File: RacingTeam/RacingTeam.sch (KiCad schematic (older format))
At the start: 68 parts, among them J1 BusIn, J2 PCB OUT, J3 Shutdown Circuit, J5 PreCharge Relay Out, J6 AIR, J7 AIR, J8 Precharge Relay, J9 Discharge Relay, Q1 2N7002, Q2 TP0610T, Q3 2N7002, Q4 TP0610T, Q5 TP0610T, Q6 2N7002, U1 LM311, U11 GLV-, U12 GLV+, U2 4N35, U3 NE555D, U4 GLV+, U5 GLV-, U6 GLV+, U6 LM311, U7 GLV-, U8 GLV-, U9 GLV-

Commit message: Update SPAN02A12.kicad_mod, EC3SAW.STEP, and 8 more files...
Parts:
- removed F1: 1000V 5A, symbol Device:Fuse
- removed J3: Shutdown Circuit, symbol Connector_Generic:Conn_01x02
- removed J8: Precharge Relay, symbol Connector_Generic:Conn_01x02
- removed J9: Discharge Relay, symbol Connector_Generic:Conn_01x02
- removed PS1: SPAN02A-12, Footprints:SPAN02A12, symbol RacingTeamPCB:SPAN02A-12
- removed R24: 2kΩ, Footprints:R_0603_1608Metric, symbol RacingTeamPCB:R
- removed R?: 100Ω, Footprints:R_0603_1608Metric, symbol RacingTeamPCB:R
- added D4, D5, D6: Flyback, symbol Device:D
- added D7: 12V, symbol RacingTeamPCB:D_Zener
- added D7: LED, symbol RacingTeamPCB:LED
- added J3, J4, J8, J9: Conn_01x01, symbol Connector_Generic:Conn_01x01
- added PS1: EC3SAW-24S12P, symbol RacingTeamPCB:EC3SAW-24S12P
- added Q7, Q8: 2N7002, symbol RacingTeamPCB:2N7000
- added R13: 1.2kΩ, symbol RacingTeamPCB:R
- added R18: 22kΩ, symbol RacingTeamPCB:R
- added R28, R29, R30: 0Ω, symbol RacingTeamPCB:R
- added U10: GLV-, symbol RacingTeamPCB:GLV-
- C1, C2, C3, C4, C5, C6, C7, C8: footprint Footprints:C_0603_1608Metric -> (none)
- J6: value AIR -> AIROut
- J7: value AIR -> Discharge Relay Out
- Q1, Q2, Q3, Q4, Q5, Q6: footprint Package_TO_SOT_SMD:SOT-23 -> (none)
- R1, R10, R11, R2, R3, R4, R5, R6, R7, R8, R9: footprint Footprints:R_0603_1608Metric -> (none)
- R12, R25: renamed from R23; footprint Footprints:R_0603_1608Metric -> (none)
- R14: renamed from R12; footprint Footprints:R_0603_1608Metric -> (none)
- R15: renamed from R13; footprint Footprints:R_0603_1608Metric -> (none)
- R16: renamed from R14; footprint Footprints:R_0603_1608Metric -> (none)
- R17: renamed from R15; footprint Footprints:R_0603_1608Metric -> (none)
- R19: renamed from R16; footprint Footprints:R_0603_1608Metric -> (none)
- R20: renamed from R17; footprint Footprints:R_0603_1608Metric -> (none)
- R21: renamed from R20; footprint Footprints:R_0603_1608Metric -> (none)
- R22: renamed from R21; footprint Footprints:R_0603_1608Metric -> (none)
- R23: renamed from R18; footprint Footprints:R_0603_1608Metric -> (none)
- R24: renamed from R19; footprint Footprints:R_0603_1608Metric -> (none)
- R26: renamed from R24; footprint Footprints:R_0603_1608Metric -> (none)
- R27: renamed from R22; footprint Footprints:R_0603_1608Metric -> (none)
- U1: footprint Footprints:TSSOP-8 -> (none)
- U2: footprint Footprints:4N35PDIP-SMD -> (none)
- U3: footprint Footprints:SOIC-8_3.9x4.9mm_P1.27mm -> (none)
- gave numbers to parts that had none: 2
- renumbered U6 to U20
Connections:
- net labels added: AIROR, PreChargeOR
- net labels removed: Discharge+, Discharge-, PrechargeIn
- wire segments 165 -> 173
- no-connect marks 4 -> 3
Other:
- note added: "12V+ - Unconverted 12V from Battery\nVCC - Diode Filtered GLV+\nGLV+ - Grounded Low Voltage +\nGLV- - Grounded Low Voltage -"
- note added: "Discharge Control\n"
- note added: "Drain\nGate\nSource"
- note added: "If=10mA"
- note added: "PreCharge Control\n\n"
- note added: "Source\nGate\nDrain\n"
- note removed: "Discharge"
- note removed: "Logic\n1. Shutdown Circuit Open Car On = Precharge Relay Open\n2. Shutdown Circuit Open Car Off = Precharge Relay Open\n3. Shutdown Circuit Closed Car Off = Precharge Relay Open\n4. Shutdown Circuit Closed Car On = Precharge Relay Closed"
- note removed: "PreCharge and Discharge (Control Side)\n"
- note removed: "Precharge and Discharge Relay (Drive Side)\n"
- note removed: "Shutdown Initiation"
- moved on the sheet: D3, J2, J5, J6, Q5, Q6

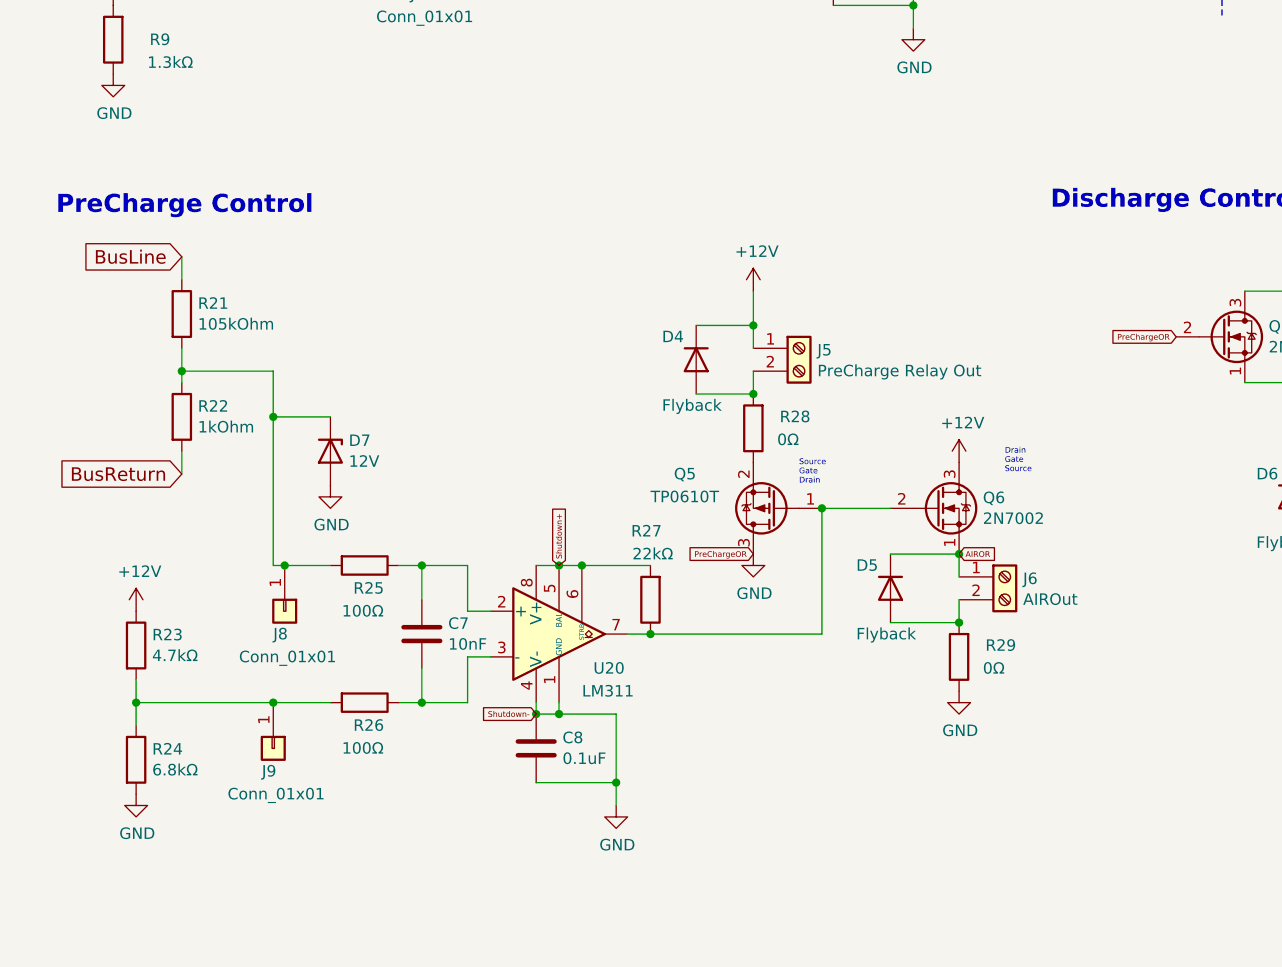
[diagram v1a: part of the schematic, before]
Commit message: Update RacingTeam.zip, PCBBom.xlsx, and 2 more files...
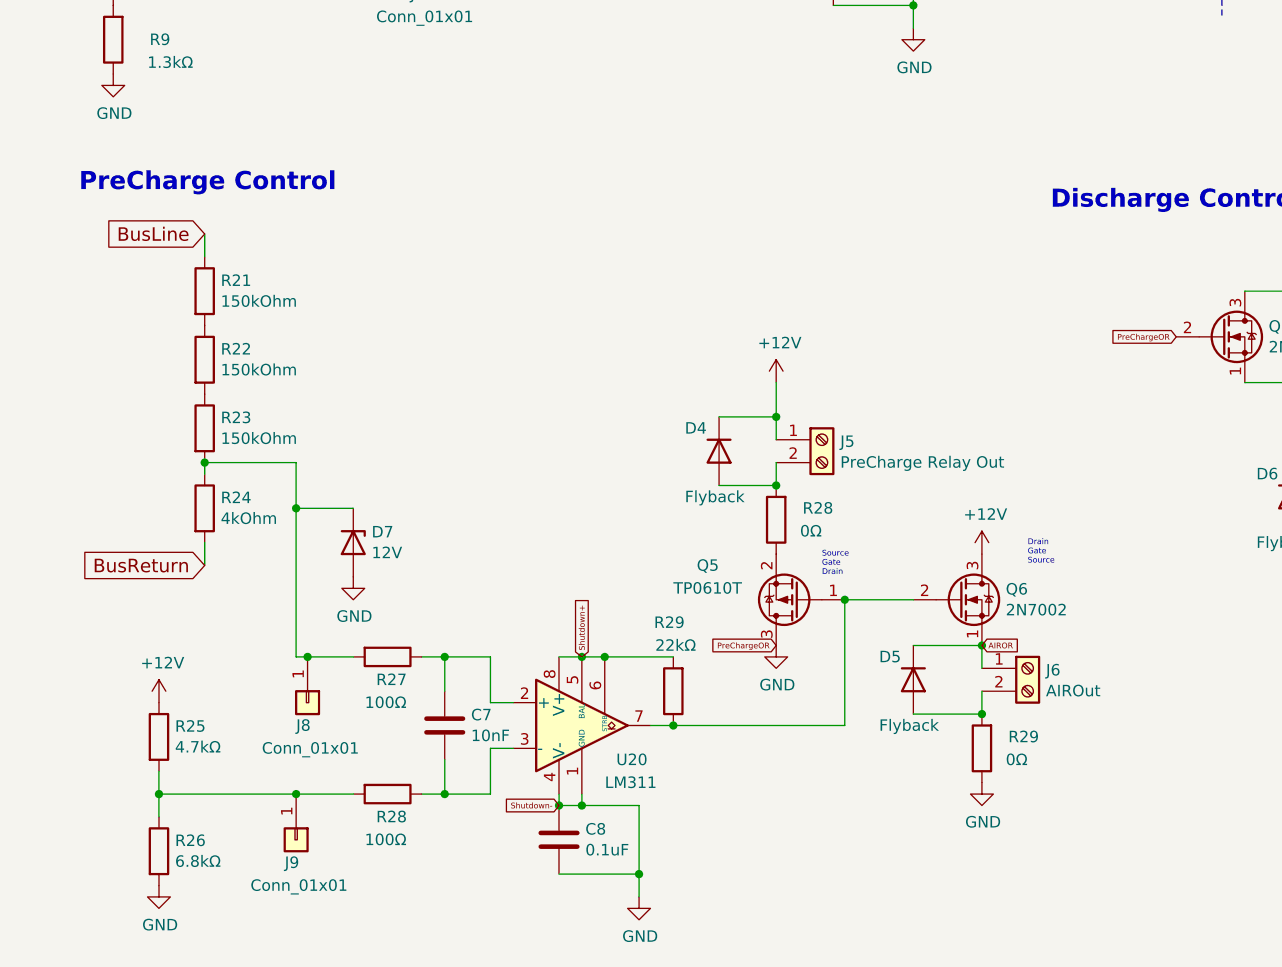
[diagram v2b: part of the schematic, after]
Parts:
- added R22, R23: 150kOhm, symbol Device:R
- R21: value 105kOhm -> 150kOhm
- R24: renamed from R22; value 1kOhm -> 4kOhm
- renumbered R23 to R25, R24 to R26, R25 to R27, R26 to R28, R27 to R29
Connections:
- net at D7.1 (K), J8.1 (Pin_1), R24.1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: now also R23.2; no longer R21.2
- new net: R21.2, R22.1
- new net: R22.2, R23.1
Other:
- moved on the sheet: C7, C8, D4, D5, D7, J5, J6, J8, J9, Q5, Q6, R21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
